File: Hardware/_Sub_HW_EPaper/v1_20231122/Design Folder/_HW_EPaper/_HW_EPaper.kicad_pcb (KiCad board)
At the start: 2 copper layers, 49.5 x 49.5 mm, 89 parts, among them J1001 USB_microB_RA, J1002 HDR_2POS_VERT, J1101 HDR_2POS_VERT, J1102 HDR_2POS_VERT, J301 HDR_4POS_VERT, J501 HDR_8POS_RA, J701 FPC_24POS_BOTTOM_0.5P, Q1001 SSM3J117TU,LF, Q701 AS3400, Q702 SSM3J117TU,LF, SW801 SPST-NO, SW802 SPST-NO, U1001 RT9526AGE, U301 PIC16F15223_8BIT, U401 W25Q64JVSSIQ, U501 SN74HCS32PWR, U601 74VHC164FT, U901 MCP9700T-E/TT

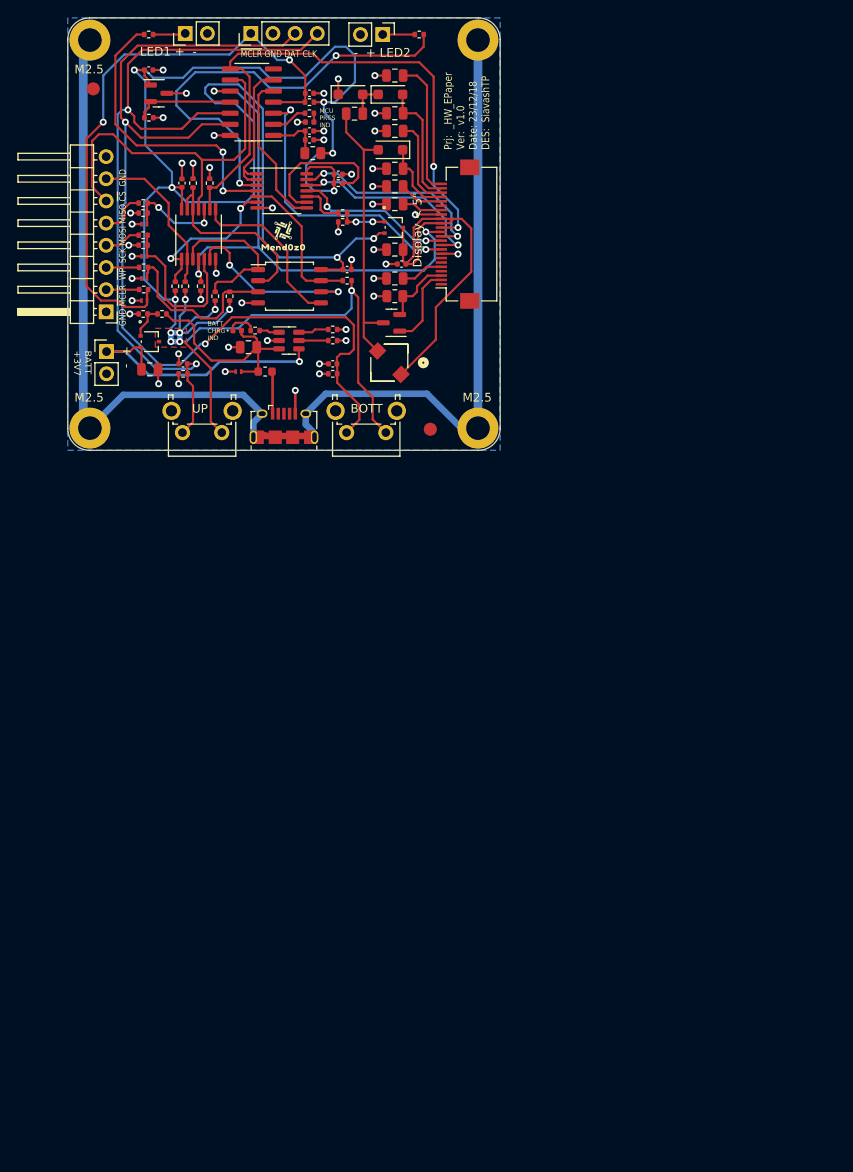
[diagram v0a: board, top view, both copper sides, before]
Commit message: Updating file templates and structures...
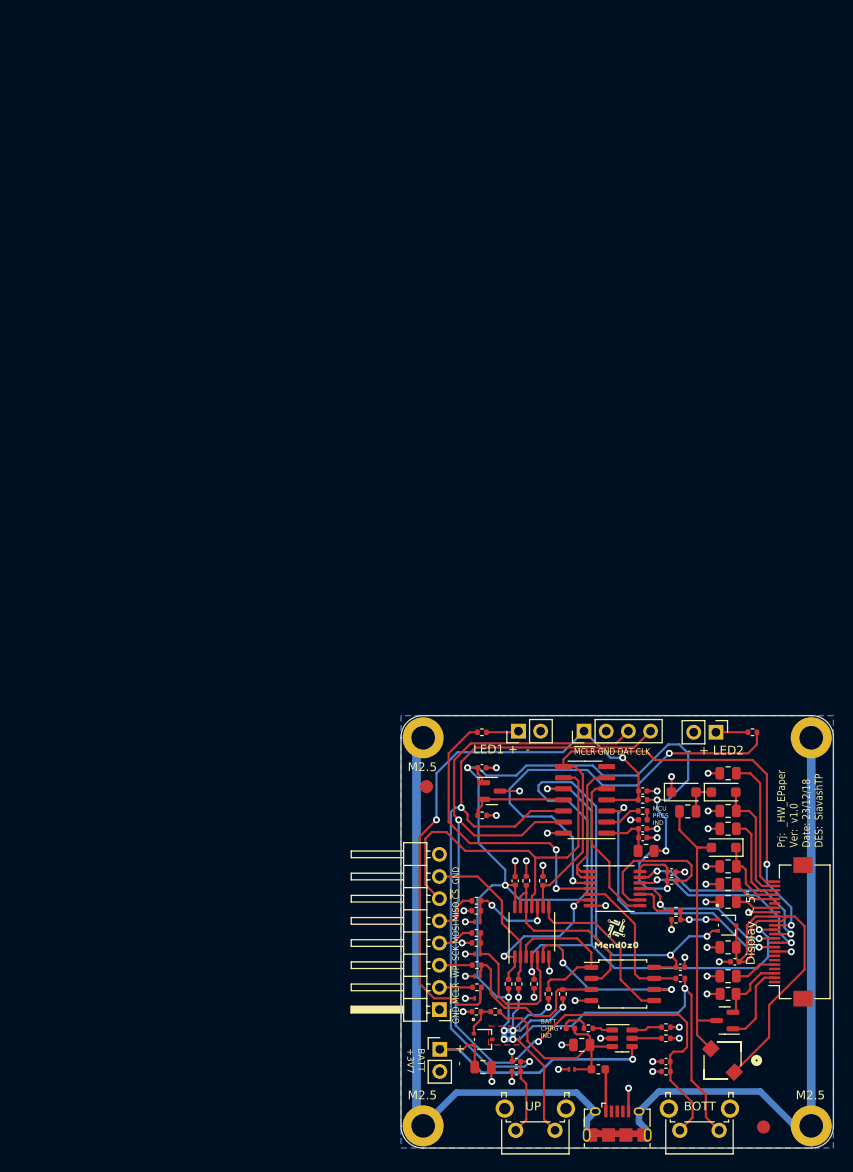
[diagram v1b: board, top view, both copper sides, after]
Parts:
- moved C1001 88.6 mm to (149.2, 234.5)
- moved C1002 88.6 mm to (160.5, 231.9)
- moved C601 88.6 mm to (170.8, 212.1)
- moved C702 88.6 mm to (177.2, 220.8)
- moved C703 88.6 mm to (178.0, 222.4)
- moved C704 88.6 mm to (177.2, 215.6)
- moved C705 88.6 mm to (177.2, 211.5)
- moved C708 88.6 mm to (172.6, 205.2)
- moved C709 88.6 mm to (177.2, 200.8)
- moved C801 88.6 mm to (170.1, 233.8)
- moved C802 88.6 mm to (153.0, 233.8)
- moved C901 88.6 mm to (149.0, 200.2)
- moved D1001 88.6 mm to (159.3, 234.7)
- moved D501 88.6 mm to (148.5, 221.5)
- moved D502 88.6 mm to (148.5, 217.8)
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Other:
- board text removed: "PCB Layout"
- board text removed: "PRELIMINARY"

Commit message: Updating Hardware File structures
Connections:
- net /BLOCK DIAGRAM/BATTERY CIRCUIT/RT_BATT renamed /BLOCK DIAGRAM/BATTERY CHARGER/RT_BATT
- net /BLOCK DIAGRAM/BATTERY CIRCUIT/RT_CHG_SB renamed /BLOCK DIAGRAM/BATTERY CHARGER/RT_CHG_SB
- net /BLOCK DIAGRAM/BATTERY CIRCUIT/RT_IMIN renamed /BLOCK DIAGRAM/BATTERY CHARGER/RT_IMIN
- net /BLOCK DIAGRAM/BATTERY CIRCUIT/RT_ISET renamed /BLOCK DIAGRAM/BATTERY CHARGER/RT_ISET
- net /BLOCK DIAGRAM/BATTERY CIRCUIT/VBUS renamed /BLOCK DIAGRAM/BATTERY CHARGER/VBUS
- net /BLOCK DIAGRAM/BATTERY CIRCUIT/V_BATT renamed /BLOCK DIAGRAM/BATTERY CHARGER/V_BATT
- net /BLOCK DIAGRAM/MCU/IND_LED renamed /BLOCK DIAGRAM/MICROCONTROLLER/IND_LED
- net /BLOCK DIAGRAM/MCU/PIC_ICSPCLK renamed /BLOCK DIAGRAM/MICROCONTROLLER/PIC_ICSPCLK
- net /BLOCK DIAGRAM/MCU/PIC_ICSPDAT renamed /BLOCK DIAGRAM/MICROCONTROLLER/PIC_ICSPDAT
- net /BLOCK DIAGRAM/MCU/PIC_~{MCLR} renamed /BLOCK DIAGRAM/MICROCONTROLLER/PIC_~{MCLR}
- net /BLOCK DIAGRAM/MCU/SIPO_CLK renamed /BLOCK DIAGRAM/MICROCONTROLLER/SIPO_CLK
- net /BLOCK DIAGRAM/MCU/SIPO_DATA renamed /BLOCK DIAGRAM/MICROCONTROLLER/SIPO_DATA
- net /BLOCK DIAGRAM/MCU/TEMP_ADC renamed /BLOCK DIAGRAM/MICROCONTROLLER/TEMP_ADC
- net /BLOCK DIAGRAM/SIPO/74VHC164_~{CLR} renamed /BLOCK DIAGRAM/SHIFT REGISTER (SIPO)/74VHC164_~{CLR}
